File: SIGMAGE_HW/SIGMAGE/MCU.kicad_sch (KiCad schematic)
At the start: 51 parts, among them J5 TSW10607GS, U15 STM32F407VGTx, X1 STDCSU18M

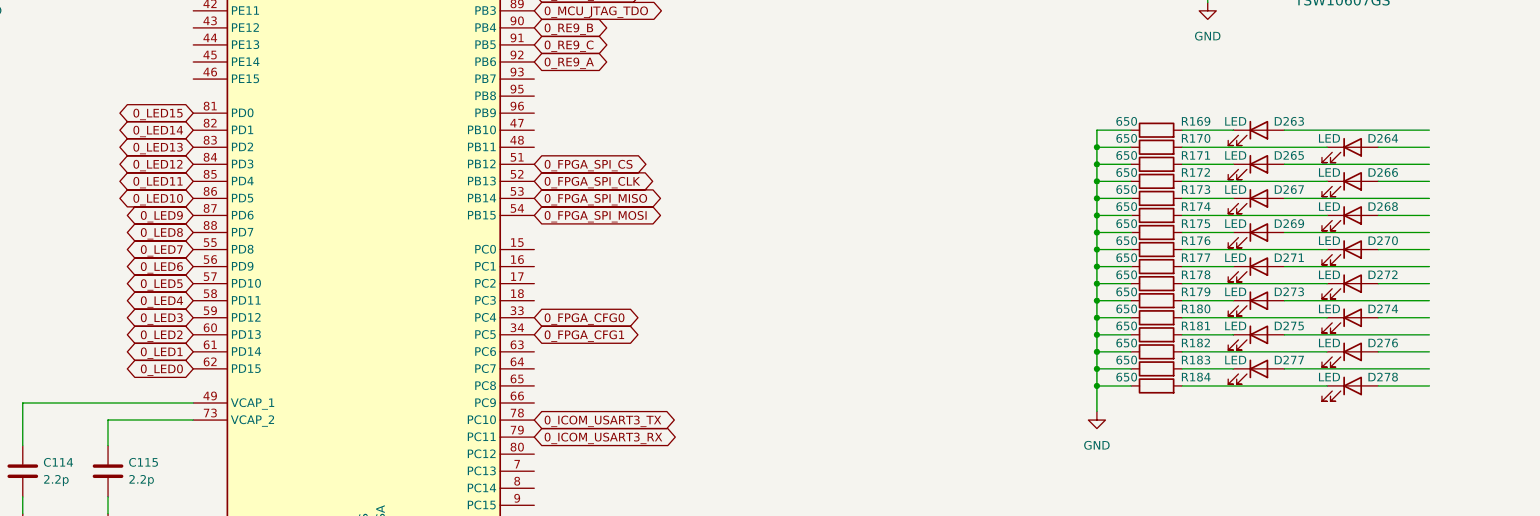
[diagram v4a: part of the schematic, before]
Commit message: some more power stuff
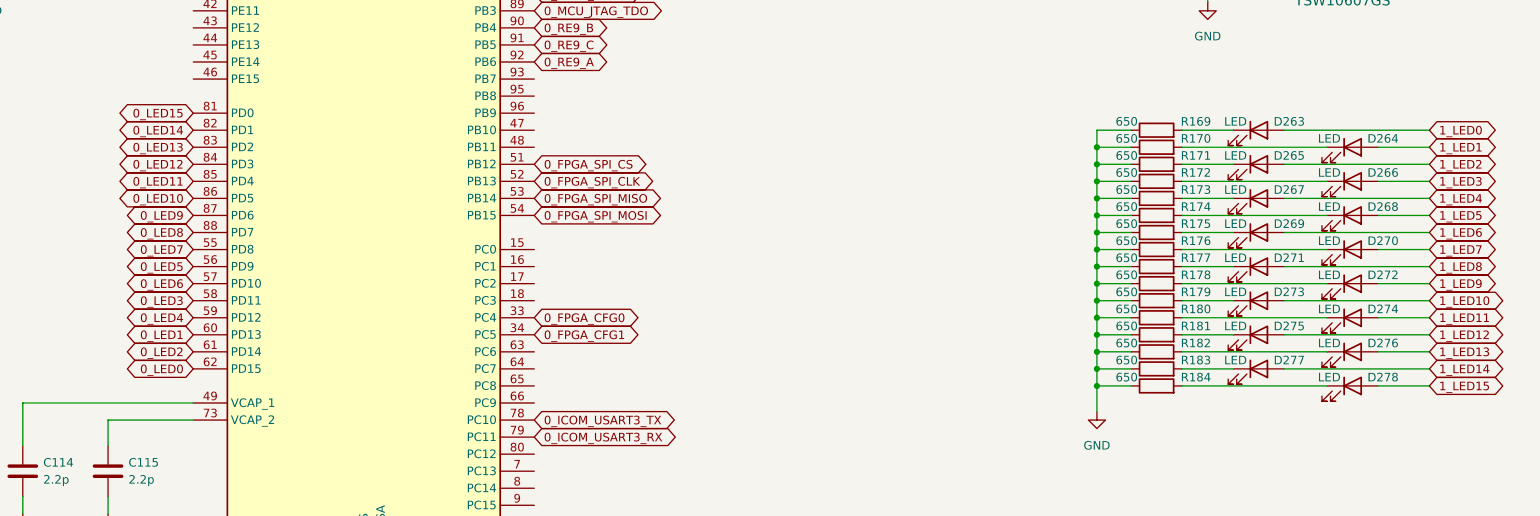
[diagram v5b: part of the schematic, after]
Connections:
- net 0_LED1: now also U15.60 (PD13); no longer U15.61 (PD14)
- net 0_LED2: now also U15.61 (PD14); no longer U15.60 (PD13)
- net 0_LED3: now also U15.58 (PD11); no longer U15.59 (PD12)
- net 0_LED4: now also U15.59 (PD12); no longer U15.58 (PD11)
- net 0_LED5: now also U15.56 (PD9); no longer U15.57 (PD10)
- net 0_LED6: now also U15.57 (PD10); no longer U15.56 (PD9)
- net 1_LED9: now reaches D272.2 (A)
- net 1_LED7: now reaches D270.2 (A)
- net 1_LED14: now reaches D277.2 (A)
- net 1_LED13: now reaches D276.2 (A)
- net 1_LED6: now reaches D269.2 (A)
- net 1_LED3: now reaches D266.2 (A)
- net 1_LED5: now reaches D268.2 (A)
- net 1_LED15: now reaches D278.2 (A)
- net 1_LED10: now reaches D273.2 (A)
- net 1_LED12: now reaches D275.2 (A)
- net 1_LED2: now reaches D265.2 (A)
- net 1_LED1: now reaches D264.2 (A)
- net 1_LED4: now reaches D267.2 (A)
- net 1_LED11: now reaches D274.2 (A)
- net 1_LED0: now reaches D263.2 (A)
- net 1_LED8: now reaches D271.2 (A)
